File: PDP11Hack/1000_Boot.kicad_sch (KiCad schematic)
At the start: 22 parts, among them SW6 Boot Vector, U1 74HCT04, U10_1 74HC74, U11_2 74HCT00, U22 74HCT138, U23 74LS240

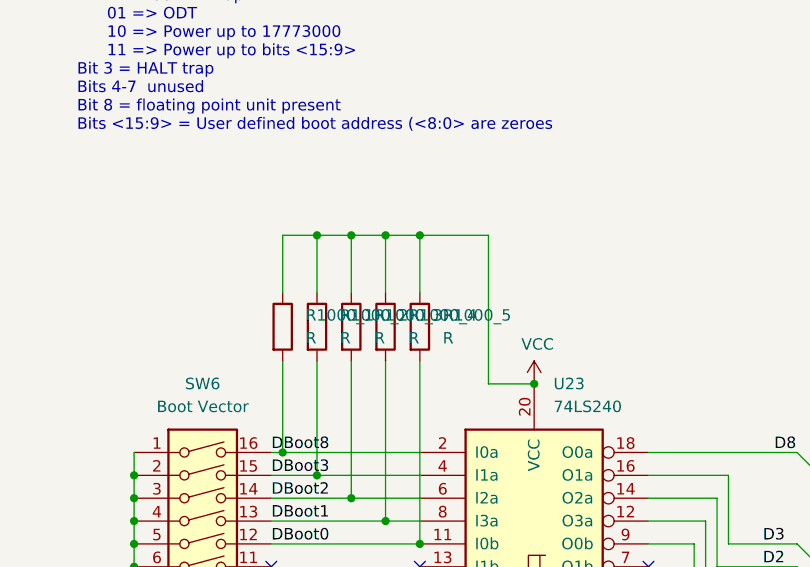
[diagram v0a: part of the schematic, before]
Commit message: Last update, PCB creation ready
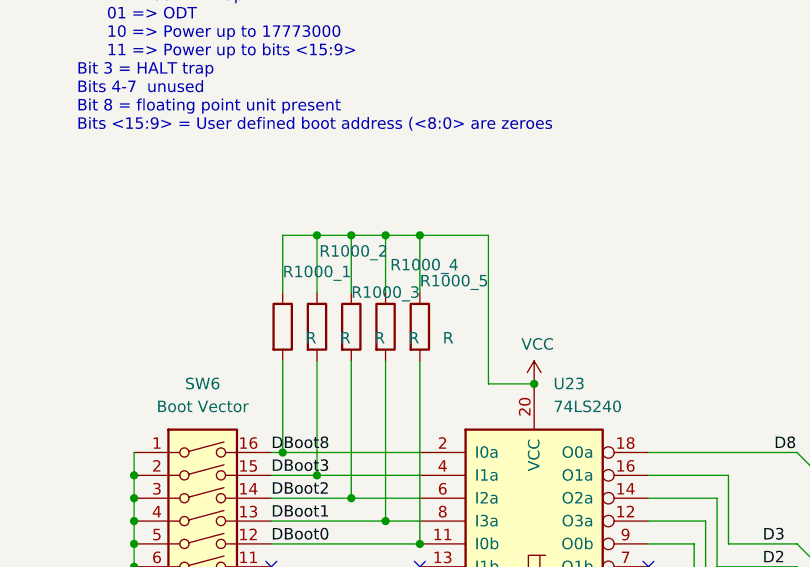
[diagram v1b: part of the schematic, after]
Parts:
- R1000_1, R1000_2, R1000_3, R1000_4, R1000_5: footprint (none) -> Resistor_THT:R_Axial_DIN0204_L3.6mm_D1.6mm_P7.62mm_Horizontal
- U1, U10_1, U11_2: footprint (none) -> Package_DIP:DIP-14_W7.62mm
- U22: footprint (none) -> Package_DIP:DIP-16_W7.62mm
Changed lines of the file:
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@@
 			)
 		)
-		(property "Footprint" ""
+		(property "Footprint" "Package_DIP:DIP-14_W7.62mm"
 			(at 60.96 86.36 0)
 			(effects
@@
 			)
 		)
-		(property "Footprint" ""
+		(property "Footprint" "Package_DIP:DIP-14_W7.62mm"
 			(at 111.76 116.84 0)
 			(effects
@@
 			)
 		)
-		(property "Footprint" ""
+		(property "Footprint" "Package_DIP:DIP-16_W7.62mm"
 			(at 44.45 124.46 0)
 			(effects
@@
 		(on_board yes)
 		(dnp no)
-		(fields_autoplaced yes)
 		(property "Reference" "R1000_5"
-			(at 181.61 88.9 0)
+			(at 179.07 85.09 0)
 			(effects
 				(font
@@
 			)
 		)
-		(property "Footprint" ""
+		(property "Footprint" "Resistor_THT:R_Axial_DIN0204_L3.6mm_D1.6mm_P7.62mm_Horizontal"
 			(at 177.292 90.17 90)
 			(effects
@@
 			)
 		)
-		(property "Footprint" ""
+		(property "Footprint" "Package_DIP:DIP-14_W7.62mm"
 			(at 134.62 175.26 0)
 			(effects
@@
 		(on_board yes)
 		(dnp no)
-		(fields_autoplaced yes)
 		(property "Reference" "R1000_1"
-			(at 166.37 88.9 0)
+			(at 163.83 84.074 0)
 			(effects
 				(font
@@
 			)
 		)
-		(property "Footprint" ""
+		(property "Footprint" "Resistor_THT:R_Axial_DIN0204_L3.6mm_D1.6mm_P7.62mm_Horizontal"
 			(at 162.052 90.17 90)
 			(effects
@@
 			)
 		)
-		(property "Footprint" ""
+		(property "Footprint" "Package_DIP:DIP-14_W7.62mm"
 			(at 83.82 119.38 0)
 			(effects
@@
 			)
 		)
-		(property "Footprint" ""
+		(property "Footprint" "Package_DIP:DIP-14_W7.62mm"
 			(at 60.96 68.58 0)
 			(effects
@@
 		(on_board yes)
 		(dnp no)
-		(fields_autoplaced yes)
 		(property "Reference" "R1000_2"
-			(at 170.18 88.9 0)
+			(at 167.894 81.788 0)
 			(effects
 				(font
@@
 			)
 		)
-		(property "Footprint" ""
+		(property "Footprint" "Resistor_THT:R_Axial_DIN0204_L3.6mm_D1.6mm_P7.62mm_Horizontal"
 			(at 165.862 90.17 90)
 			(effects
@@
 		(on_board yes)
 		(dnp no)
-		(fields_autoplaced yes)
 		(property "Reference" "R1000_3"
-			(at 173.99 88.9 0)
+			(at 171.45 86.36 0)
 			(effects
 				(font
@@
 			)
 		)
-		(property "Footprint" ""
+		(property "Footprint" "Resistor_THT:R_Axial_DIN0204_L3.6mm_D1.6mm_P7.62mm_Horizontal"
 			(at 169.672 90.17 90)
 			(effects
@@
 			)
 		)
-		(property "Footprint" ""
+		(property "Footprint" "Package_DIP:DIP-14_W7.62mm"
 			(at 83.82 101.6 0)
 			(effects
@@
 			)
 		)
-		(property "Footprint" ""
+		(property "Footprint" "Package_DIP:DIP-14_W7.62mm"
 			(at 114.3 175.26 0)
 			(effects
@@
 		(on_board yes)
 		(dnp no)
-		(fields_autoplaced yes)
 		(property "Reference" "R1000_4"
-			(at 177.8 88.9 0)
+			(at 175.768 83.312 0)
 			(effects
 				(font
@@
 			)
 		)
-		(property "Footprint" ""
+		(property "Footprint" "Resistor_THT:R_Axial_DIN0204_L3.6mm_D1.6mm_P7.62mm_Horizontal"
 			(at 173.482 90.17 90)
 			(effects
